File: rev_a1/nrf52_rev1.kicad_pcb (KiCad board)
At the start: 2 copper layers, 48.3 x 48.3 mm, 31 parts, among them P1 CONN_01X18, P2 CONN_01X18, P3 USB_OTG, U1 nRF52832, U2 CP2102, U3 LT1129CST-3.3, Y1 32K, Y2 32M

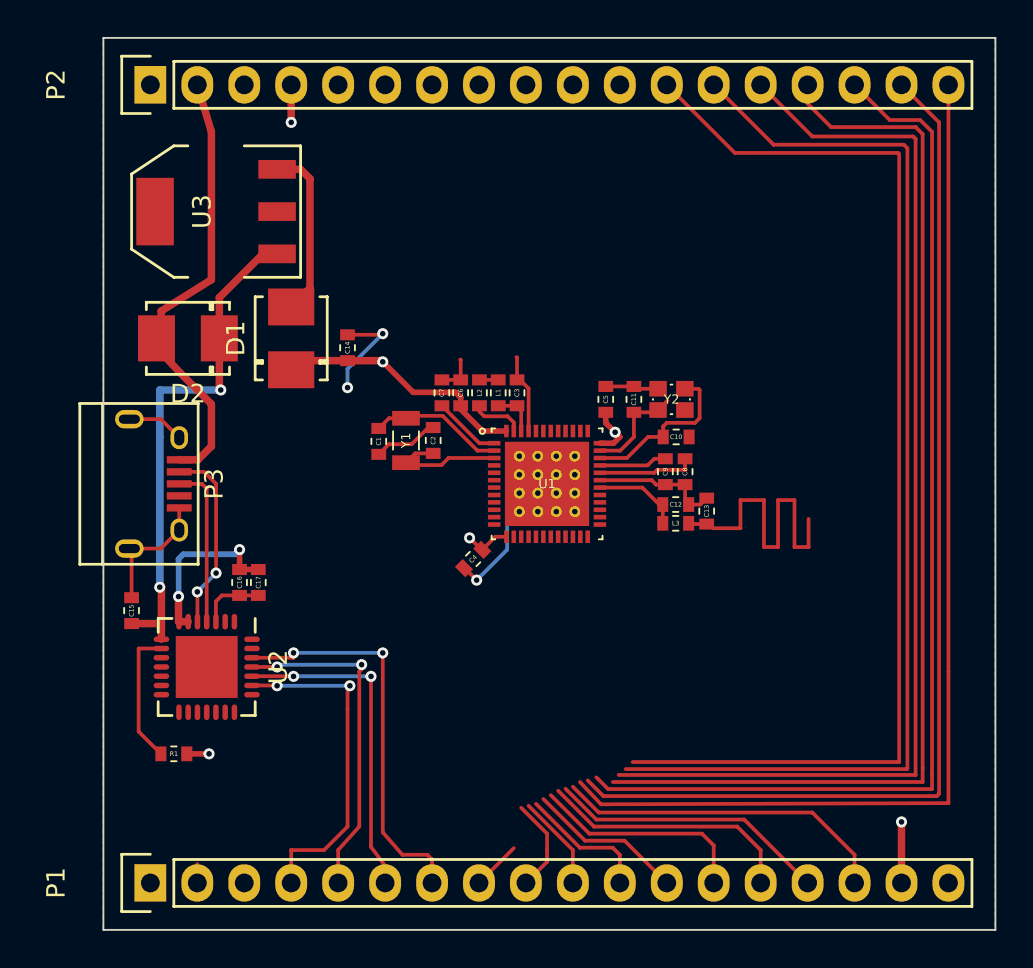
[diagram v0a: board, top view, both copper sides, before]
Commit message: wip
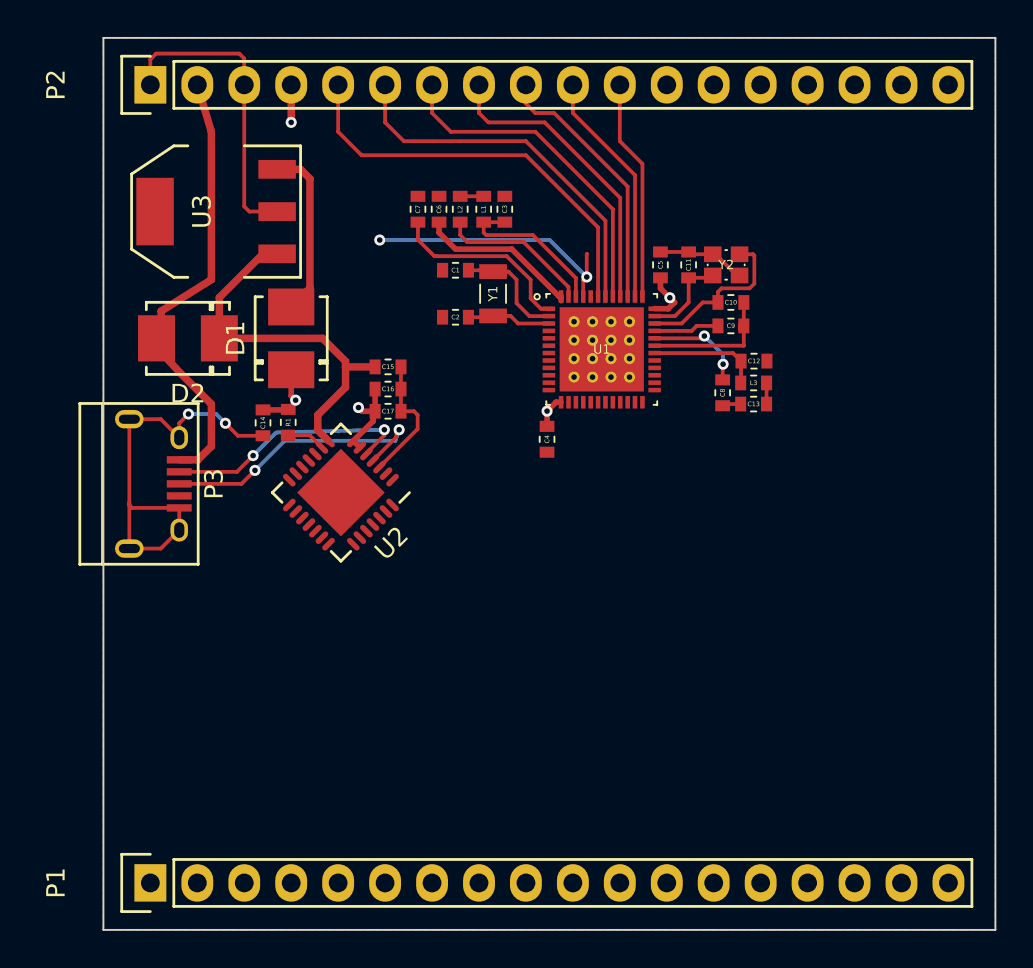
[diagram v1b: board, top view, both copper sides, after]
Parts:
- moved C15 19.1 mm to (40.8, 43.2), turned to 180 degrees
- moved R1 19.0 mm to (35.4, 46.2), turned to 90 degrees
- moved C16 13.2 mm to (40.8, 44.4), turned to 180 degrees
- moved U2 11.9 mm to (38.2, 50.0), turned to 225 degrees
- moved C17 11.6 mm to (40.8, 45.6), turned to 180 degrees
- moved C1 10.1 mm to (44.5, 38.0), turned to 0 degrees
- moved C7 10.0 mm to (42.4, 34.7)
- moved C6 10.00 mm to (43.6, 34.7)
- moved L2 9.99 mm to (44.7, 34.7)
- moved L1 9.96 mm to (46.0, 34.7)
- moved C3 9.95 mm to (47.1, 34.7)
- moved Y1 9.23 mm to (46.5, 39.2)
- moved C12 8.84 mm to (60.6, 42.9)
- moved L3 8.69 mm to (60.6, 44.1)
- moved C9 8.65 mm to (59.3, 41.0), turned to 0 degrees
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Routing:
- net P0.24: track 61.4 -> 0.00 mm
- net P0.23: track 60.7 -> 0.00 mm
- net P0.22: track 60.1 -> 0.00 mm
- net P0.20: track 59.3 -> 0.00 mm
- net SWDCLK: track 59.3 -> 0.10 mm
- net SWDIO: track 60.4 -> 1.65 mm
- net P0.21: track 58.6 -> 0.00 mm
- net GND: track 69.4 -> 100.7 mm, vias 3 -> 4
- net P0.31: track 0.00 -> 23.2 mm
- net P0.08: track 21.6 -> 0.00 mm, vias 2 -> 0
- net P0.30: track 0.00 -> 20.3 mm
- net P0.05: track 18.3 -> 0.00 mm, vias 2 -> 0
- net P0.06: track 18.3 -> 0.00 mm, vias 2 -> 0
- net P0.19: track 18.3 -> 0.00 mm
- net P0.29: track 0.00 -> 18.2 mm
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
